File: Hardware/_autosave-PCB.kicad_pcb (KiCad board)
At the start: 2 copper layers, 53.4 x 22 mm, 9 parts, among them J1 Conn_01x04_Pin, U1 ME54BS01_V1.0, U2 MCP1700x-330xxTO

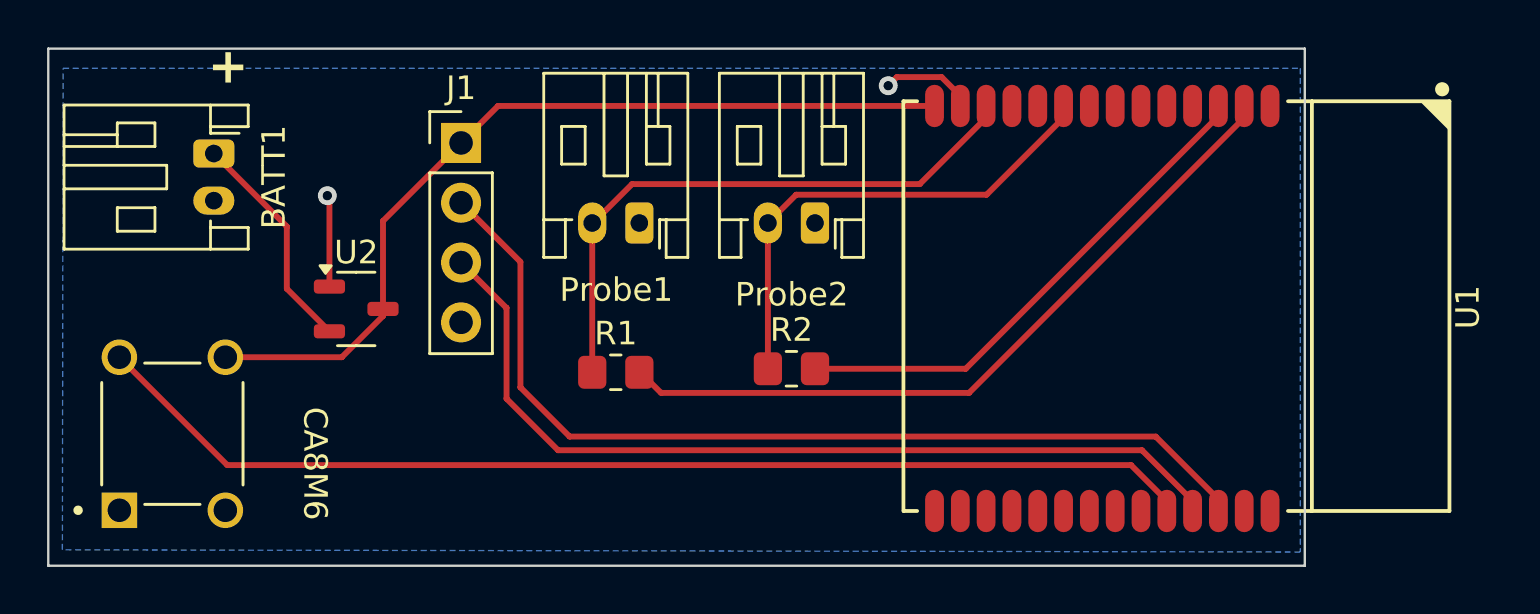
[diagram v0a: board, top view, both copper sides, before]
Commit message: Work on PCB
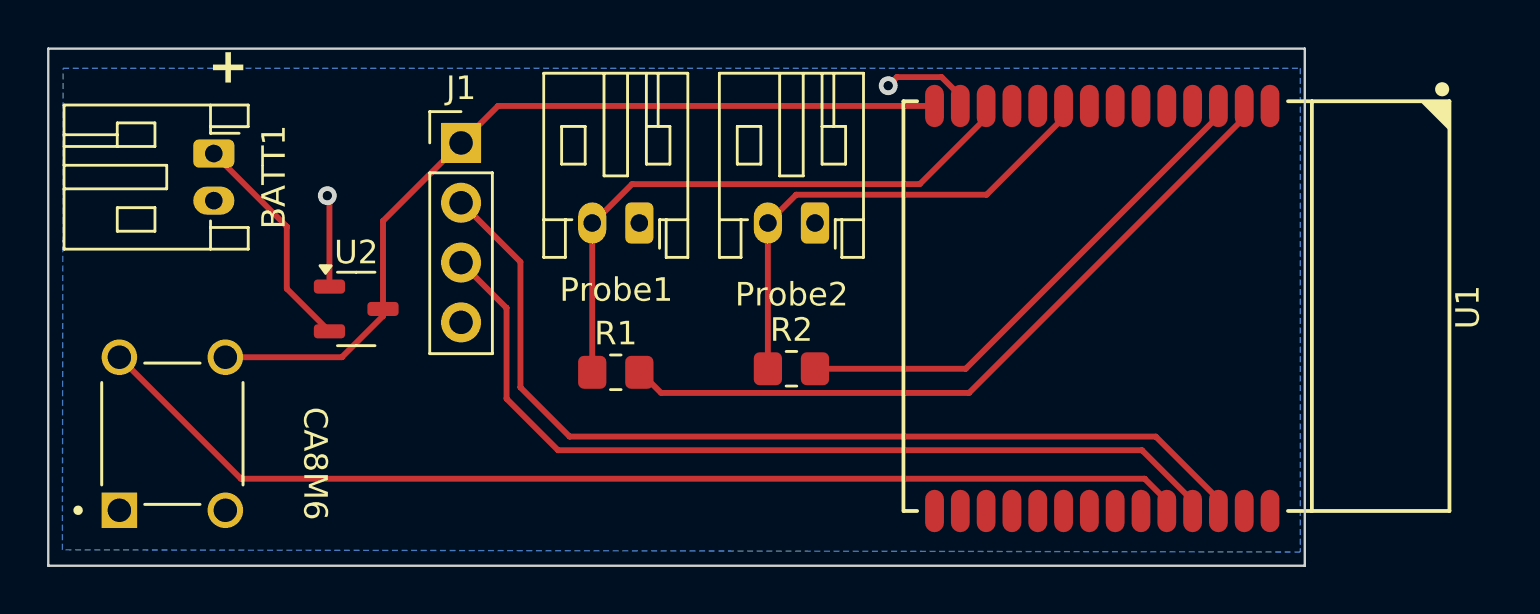
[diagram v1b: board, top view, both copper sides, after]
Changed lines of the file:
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@@
 	)
 	(segment
-		(start 48.531 72.991)
+		(start 88.43 74.94)
+		(end 88.43 74.509281)
+		(width 0.25)
+		(layer "F.Cu")
+		(net 3)
+	)
+	(segment
+		(start 49.11 73.57)
 		(end 43.95 68.41)
 		(width 0.25)
@@
 	)
 	(segment
-		(start 86.911719 72.991)
-		(end 48.531 72.991)
+		(start 88.43 74.509281)
+		(end 87.490719 73.57)
 		(width 0.25)
 		(layer "F.Cu")
@@
 	)
 	(segment
-		(start 88.43 74.509281)
-		(end 86.911719 72.991)
+		(start 87.490719 73.57)
+		(end 49.11 73.57)
 		(width 0.25)
 		(layer "F.Cu")
-		(net 3)
-	)
-	(segment
-		(start 88.43 74.94)
-		(end 88.43 74.509281)
-		(width 0.25)
-		(layer "F.Cu")
